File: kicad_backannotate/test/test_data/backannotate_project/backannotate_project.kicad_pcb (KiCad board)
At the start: 2 copper layers, 8 parts

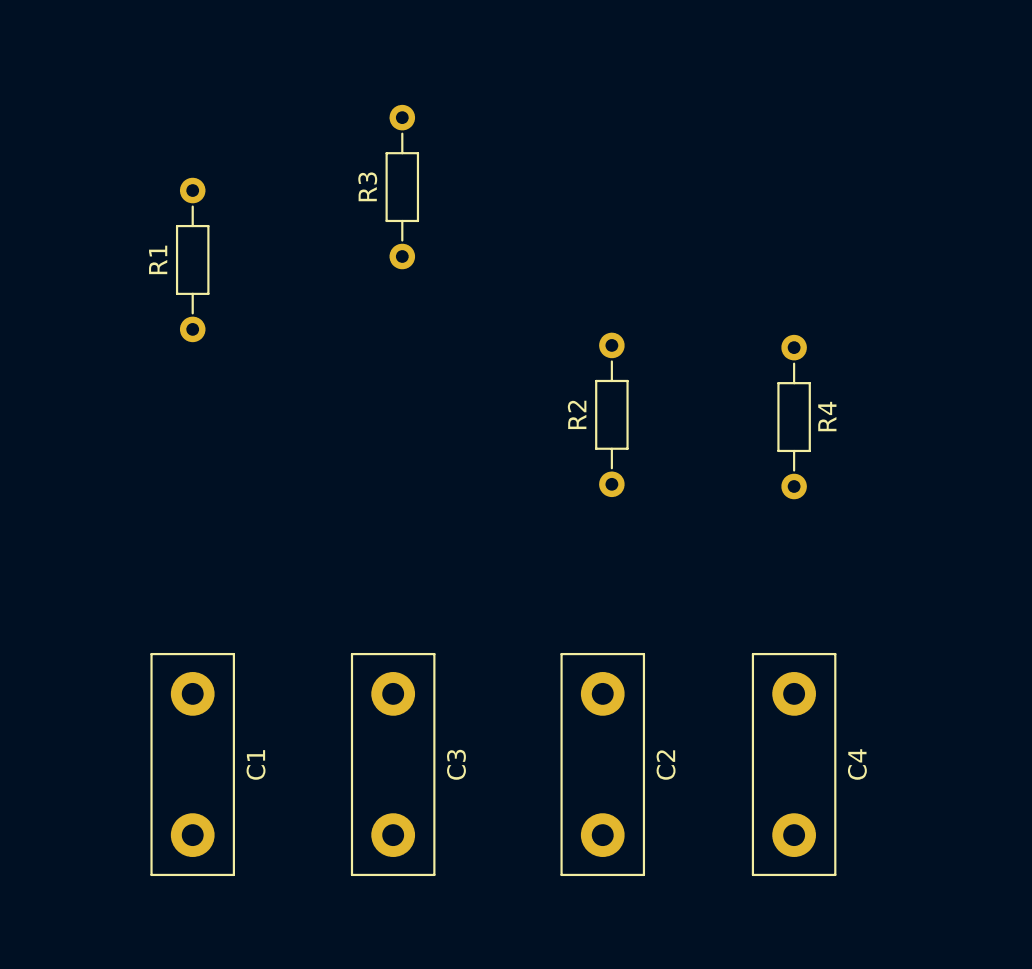
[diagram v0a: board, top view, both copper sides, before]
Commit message: docs update
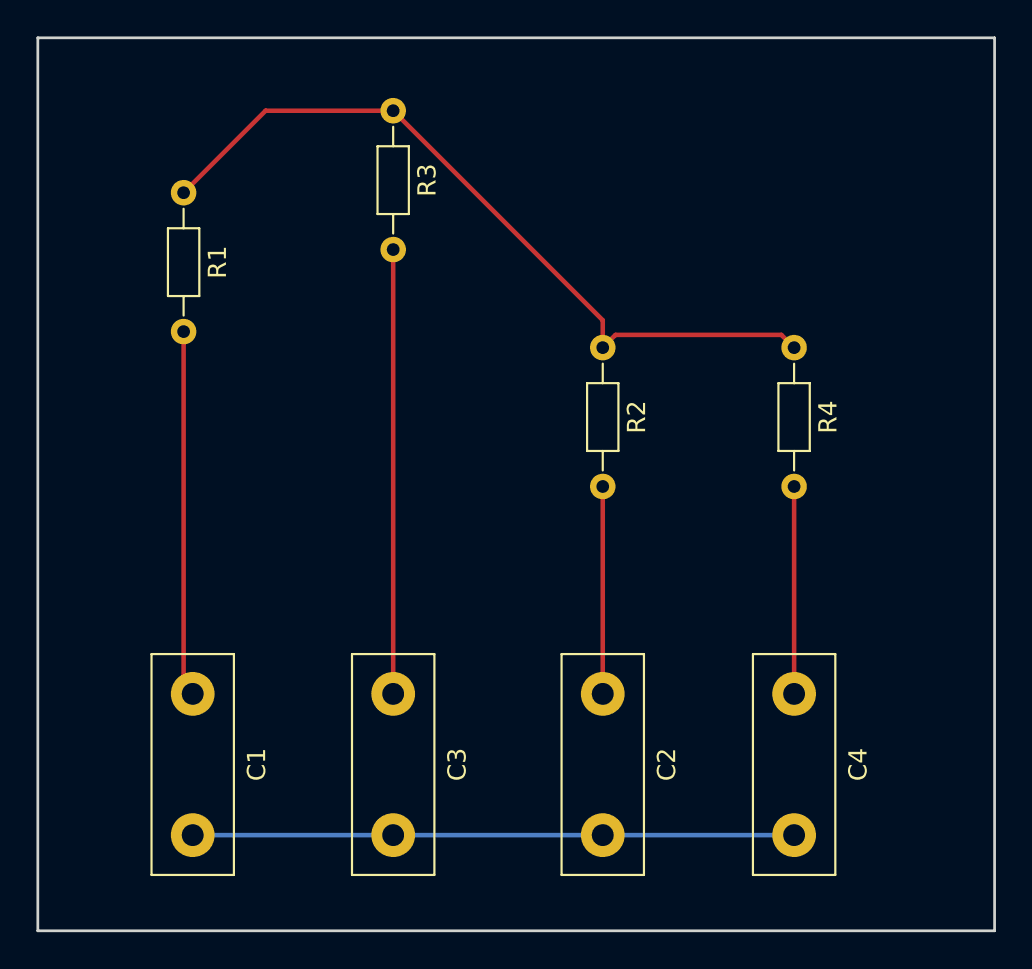
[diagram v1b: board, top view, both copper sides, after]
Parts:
- moved R3 8.02 mm to (84.0, 20.0), turned to 270 degrees
- moved R1 7.52 mm to (72.5, 24.5), turned to 270 degrees
- moved R2 7.52 mm to (95.5, 33.0), turned to 270 degrees
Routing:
- net +15V: track 0.00 -> 42.2 mm
- net GND: track 0.00 -> 33.0 mm
- net Net-(C3-Pad1): track 0.00 -> 24.4 mm
- net Net-(C1-Pad1): track 0.00 -> 20.1 mm
- net Net-(C4-Pad1): track 0.00 -> 11.4 mm
- net Net-(C2-Pad1): track 0.00 -> 11.4 mm
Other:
- board outline added: 52.5 x 49 mm
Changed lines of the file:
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@@
   (general
     (thickness 1.6)
-    (drawings 0)
-    (tracks 0)
+    (drawings 5)
+    (tracks 15)
     (zones 0)
     (modules 8)
@@
   )
   (module Resistors_THT:R_Axial_DIN0204_L3.6mm_D1.6mm_P7.62mm_Horizontal (layer F.Cu)
-    (at 73 32 90)
+    (at 72.5 24.5 270)
     (descr "Resistor, Axial_DIN0204 series, Axial, Horizontal, pin pitch=7.62mm, 0.16666666666666666W = 1/6W, length*diameter=3.6*1.6mm^2, http://cdn-reichelt.de/documents/datenblatt/B400/1_4W%23YAG.pdf")
     (tags "Resistor Axial_DIN0204 series Axial Horizontal pin pitch 7.62mm 0.16666666666666666W = 1/6W length 3.6mm diameter 1.6mm")
-    (fp_text reference R1 (at 3.81 -1.86 90) (layer F.SilkS)
-      (effects (font (size 1 1) (thickness 0.15)))
-    )
-    (fp_text value R (at 3.81 1.86 90) (layer F.Fab)
+    (fp_text reference R1 (at 3.81 -1.86 270) (layer F.SilkS)
+      (effects (font (size 1 1) (thickness 0.15)))
+    )
+    (fp_text value R (at 3.81 1.86 270) (layer F.Fab)
       (effects (font (size 1 1) (thickness 0.15)))
     )
@@
     (fp_line (start 2.01 0.8) (end 5.61 0.8) (layer F.Fab) (width 0.1))
     (fp_line (start 2.01 -0.8) (end 2.01 0.8) (layer F.Fab) (width 0.1))
-    (pad 2 thru_hole oval (at 7.62 0 90) (size 1.4 1.4) (drill 0.7) (layers *.Cu *.Mask)
+    (pad 2 thru_hole oval (at 7.62 0 270) (size 1.4 1.4) (drill 0.7) (layers *.Cu *.Mask)
       (net 2 "Net-(C1-Pad1)"))
-    (pad 1 thru_hole circle (at 0 0 90) (size 1.4 1.4) (drill 0.7) (layers *.Cu *.Mask)
+    (pad 1 thru_hole circle (at 0 0 270) (size 1.4 1.4) (drill 0.7) (layers *.Cu *.Mask)
       (net 6 +15V))
     (model ${KISYS3DMOD}/Resistors_THT.3dshapes/R_Axial_DIN0204_L3.6mm_D1.6mm_P7.62mm_Horizontal.wrl
@@
   )
   (module Resistors_THT:R_Axial_DIN0204_L3.6mm_D1.6mm_P7.62mm_Horizontal (layer F.Cu)
-    (at 96 40.5 90)
+    (at 95.5 33 270)
     (descr "Resistor, Axial_DIN0204 series, Axial, Horizontal, pin pitch=7.62mm, 0.16666666666666666W = 1/6W, length*diameter=3.6*1.6mm^2, http://cdn-reichelt.de/documents/datenblatt/B400/1_4W%23YAG.pdf")
     (tags "Resistor Axial_DIN0204 series Axial Horizontal pin pitch 7.62mm 0.16666666666666666W = 1/6W length 3.6mm diameter 1.6mm")
-    (fp_text reference R2 (at 3.81 -1.86 90) (layer F.SilkS)
-      (effects (font (size 1 1) (thickness 0.15)))
-    )
-    (fp_text value R (at 3.81 1.86 90) (layer F.Fab)
+    (fp_text reference R2 (at 3.81 -1.86 270) (layer F.SilkS)
+      (effects (font (size 1 1) (thickness 0.15)))
+    )
+    (fp_text value R (at 3.81 1.86 270) (layer F.Fab)
       (effects (font (size 1 1) (thickness 0.15)))
     )
@@
     (fp_line (start 8.6 1.15) (end 8.6 -1.15) (layer F.CrtYd) (width 0.05))
     (fp_line (start 8.6 -1.15) (end -0.95 -1.15) (layer F.CrtYd) (width 0.05))
-    (pad 1 thru_hole circle (at 0 0 90) (size 1.4 1.4) (drill 0.7) (layers *.Cu *.Mask)
+    (pad 1 thru_hole circle (at 0 0 270) (size 1.4 1.4) (drill 0.7) (layers *.Cu *.Mask)
       (net 6 +15V))
-    (pad 2 thru_hole oval (at 7.62 0 90) (size 1.4 1.4) (drill 0.7) (layers *.Cu *.Mask)
+    (pad 2 thru_hole oval (at 7.62 0 270) (size 1.4 1.4) (drill 0.7) (layers *.Cu *.Mask)
       (net 3 "Net-(C2-Pad1)"))
     (model ${KISYS3DMOD}/Resistors_THT.3dshapes/R_Axial_DIN0204_L3.6mm_D1.6mm_P7.62mm_Horizontal.wrl
@@
   )
   (module Resistors_THT:R_Axial_DIN0204_L3.6mm_D1.6mm_P7.62mm_Horizontal (layer F.Cu)
-    (at 84.5 28 90)
+    (at 84 20 270)
     (descr "Resistor, Axial_DIN0204 series, Axial, Horizontal, pin pitch=7.62mm, 0.16666666666666666W = 1/6W, length*diameter=3.6*1.6mm^2, http://cdn-reichelt.de/documents/datenblatt/B400/1_4W%23YAG.pdf")
     (tags "Resistor Axial_DIN0204 series Axial Horizontal pin pitch 7.62mm 0.16666666666666666W = 1/6W length 3.6mm diameter 1.6mm")
-    (fp_text reference R3 (at 3.81 -1.86 90) (layer F.SilkS)
-      (effects (font (size 1 1) (thickness 0.15)))
-    )
-    (fp_text value R (at 3.81 1.86 90) (layer F.Fab)
+    (fp_text reference R3 (at 3.81 -1.86 270) (layer F.SilkS)
+      (effects (font (size 1 1) (thickness 0.15)))
+    )
+    (fp_text value R (at 3.81 1.86 270) (layer F.Fab)
       (effects (font (size 1 1) (thickness 0.15)))
     )
@@
     (fp_line (start 2.01 0.8) (end 5.61 0.8) (layer F.Fab) (width 0.1))
     (fp_line (start 2.01 -0.8) (end 2.01 0.8) (layer F.Fab) (width 0.1))
-    (pad 2 thru_hole oval (at 7.62 0 90) (size 1.4 1.4) (drill 0.7) (layers *.Cu *.Mask)
+    (pad 2 thru_hole oval (at 7.62 0 270) (size 1.4 1.4) (drill 0.7) (layers *.Cu *.Mask)
       (net 4 "Net-(C3-Pad1)"))
-    (pad 1 thru_hole circle (at 0 0 90) (size 1.4 1.4) (drill 0.7) (layers *.Cu *.Mask)
+    (pad 1 thru_hole circle (at 0 0 270) (size 1.4 1.4) (drill 0.7) (layers *.Cu *.Mask)
       (net 6 +15V))
     (model ${KISYS3DMOD}/Resistors_THT.3dshapes/R_Axial_DIN0204_L3.6mm_D1.6mm_P7.62mm_Horizontal.wrl
@@
     )
   )
+  (gr_line (start 64.5 16) (end 64.5 16) (layer Edge.Cuts) (width 0.15))
+  (gr_line (start 64.5 65) (end 64.5 16) (layer Edge.Cuts) (width 0.15))
+  (gr_line (start 117 65) (end 64.5 65) (layer Edge.Cuts) (width 0.15))
+  (gr_line (start 117 16) (end 117 65) (layer Edge.Cuts) (width 0.15))
+  (gr_line (start 64.5 16) (end 117 16) (layer Edge.Cuts) (width 0.15))
+  (segment (start 95.5 59.75) (end 106 59.75) (width 0.25) (layer B.Cu) (net 1))
+  (segment (start 84 59.75) (end 95.5 59.75) (width 0.25) (layer B.Cu) (net 1))
+  (segment (start 73 59.75) (end 84 59.75) (width 0.25) (layer B.Cu) (net 1))
+  (segment (start 72.5 32.12) (end 72.5 51.5) (width 0.25) (layer F.Cu) (net 2))
+  (segment (start 72.5 51.5) (end 73 52) (width 0.25) (layer F.Cu) (net 2))
+  (segment (start 95.5 40.62) (end 95.5 52) (width 0.25) (layer F.Cu) (net 3))
+  (segment (start 84 27.62) (end 84 52) (width 0.25) (layer F.Cu) (net 4))
+  (segment (start 106 40.62) (end 106 52) (width 0.25) (layer F.Cu) (net 5))
+  (segment (start 84 20) (end 77 20) (width 0.25) (layer F.Cu) (net 6))
+  (segment (start 77 20) (end 72.5 24.5) (width 0.25) (layer F.Cu) (net 6))
+  (segment (start 95.5 33) (end 95.5 31.5) (width 0.25) (layer F.Cu) (net 6))
+  (segment (start 95.5 31.5) (end 84 20) (width 0.25) (layer F.Cu) (net 6))
+  (segment (start 106 33) (end 105.300001 32.300001) (width 0.25) (layer F.Cu) (net 6))
+  (segment (start 105.300001 32.300001) (end 96.199999 32.300001) (width 0.25) (layer F.Cu) (net 6))
+  (segment (start 96.199999 32.300001) (end 95.5 33) (width 0.25) (layer F.Cu) (net 6))
 )
